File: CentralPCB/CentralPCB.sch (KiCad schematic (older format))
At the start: 60 parts, among them J1 POWER HEADER, J2 SPI Header, J3 Conn_01x24, J4 Conn_01x24, J5 Conn_02x16_Odd_Even, J6 Conn_Coaxial, J7 Conn_02x10_Odd_Even, J8 Conn_01x05, U1 AD8531, U2 Teensy4.1, U3 BA7810CP-E2

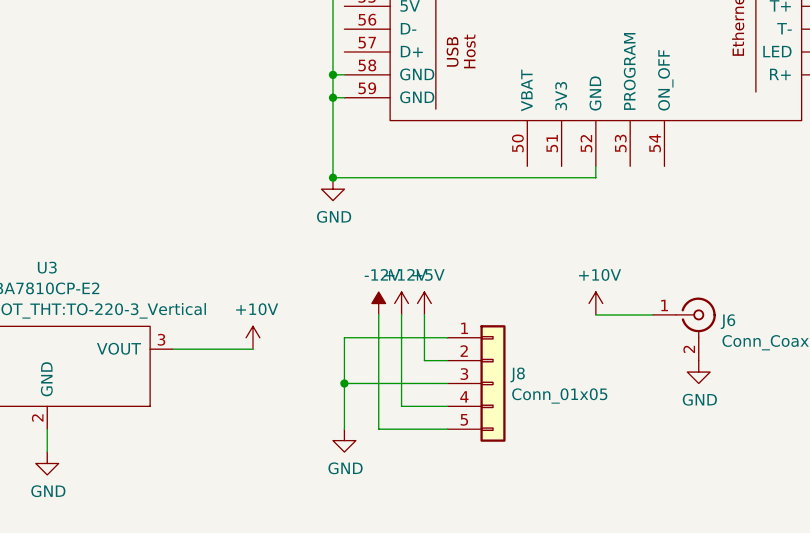
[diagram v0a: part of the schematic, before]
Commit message: More routing CentralPCB
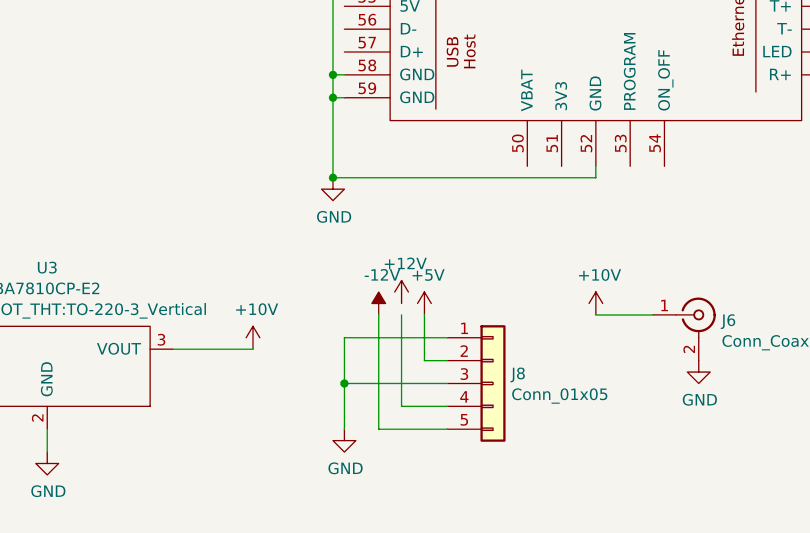
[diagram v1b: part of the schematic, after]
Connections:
- net +12V: no longer J8.4 (Pin_4)
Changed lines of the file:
@@
 	3100 7200 3550 7200
-Wire Wire Line
-	3550 7000 3100 7000
 Wire Wire Line
 	3100 7000 3100 7200
@@
 Wire Wire Line
 	3450 7100 3550 7100
-$Comp
-L power:+12V #PWR017
-U 1 1 6190D75E
-P 3350 6900
-F 0 "#PWR017" H 3350 6750 50  0001 C CNN
-F 1 "+12V" H 3365 7073 50  0000 C CNN
-F 2 "" H 3350 6900 50  0001 C CNN
-F 3 "" H 3350 6900 50  0001 C CNN
-	1    3350 6900
-	1    0    0    -1
-$EndComp
-Wire Wire Line
-	3350 6900 3350 7300
 Wire Wire Line
 	3350 7300 3550 7300
@@
 Wire Wire Line
 	850  1200 950  1200
+Wire Wire Line
+	3350 6900 3350 7300
+Wire Wire Line
+	3550 7000 3100 7000
+$Comp
+L power:+12V #PWR017
+U 1 1 6190D75E
+P 3350 6850
+F 0 "#PWR017" H 3350 6700 50  0001 C CNN
+F 1 "+12V" H 3365 7023 50  0000 C CNN
+F 2 "" H 3350 6850 50  0001 C CNN
+F 3 "" H 3350 6850 50  0001 C CNN
+	1    3350 6850
+	1    0    0    -1
+$EndComp
 $EndSCHEMATC
